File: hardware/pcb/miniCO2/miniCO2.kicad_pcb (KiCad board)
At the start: 4 copper layers, 13.7 x 28.2 mm, 12 parts, among them J1 USB_A, J2 Conn_01x04_Socket, SW1 SW_Push, U1 ATSAMD21E18A-M, U2 AP2112K-3.3, U3 SCD40-D-R2

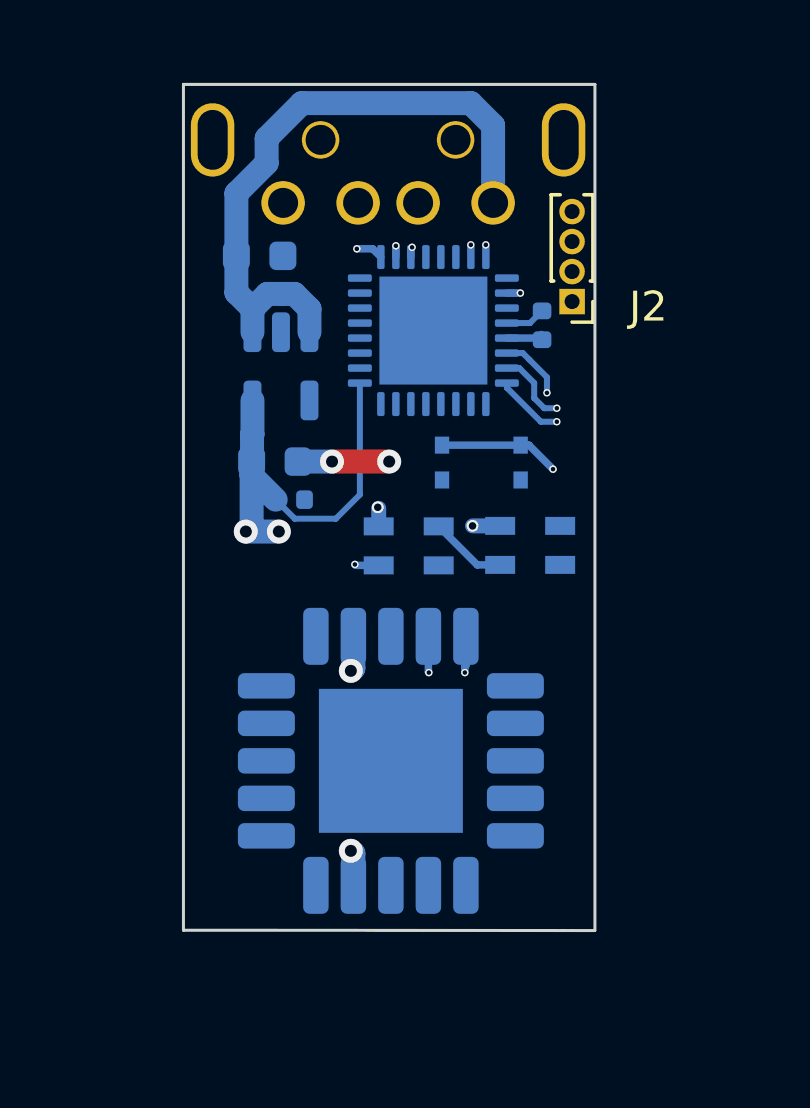
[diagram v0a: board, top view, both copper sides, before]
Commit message: Version 1 finished
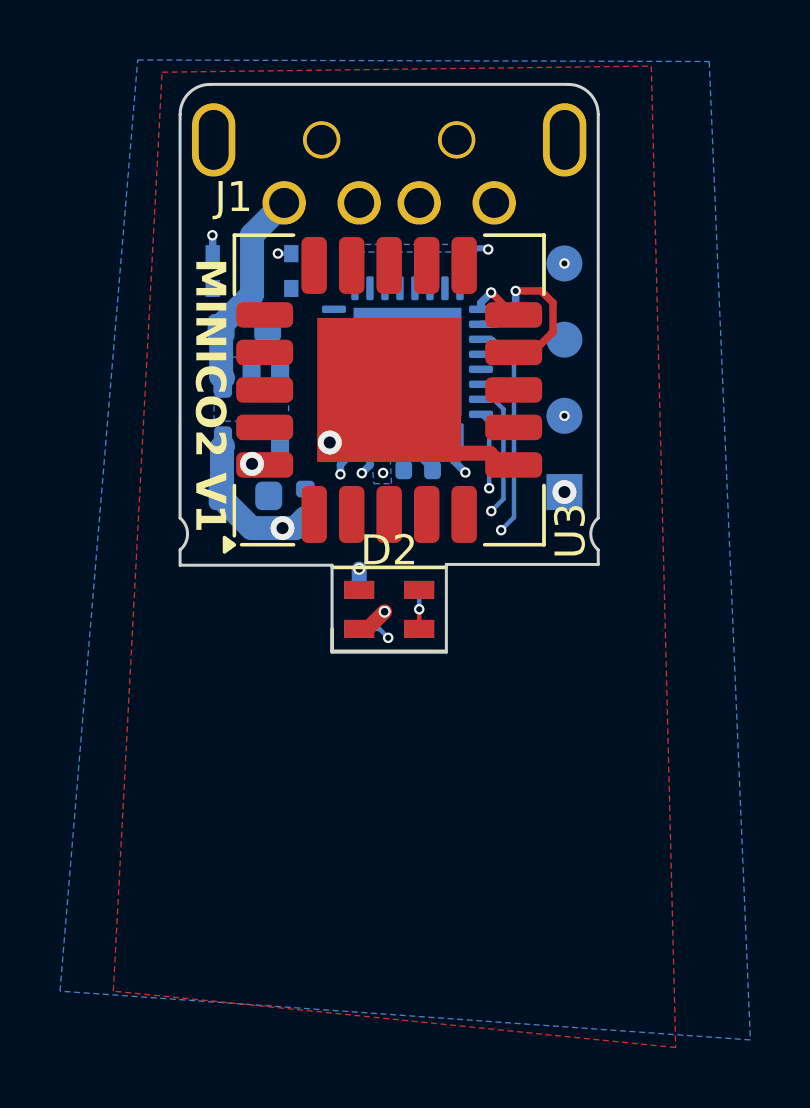
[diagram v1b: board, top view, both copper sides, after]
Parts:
- D1: footprint miniCO2:LED_SK6805_PLCC4_2.4x2.7mm_P1.3mm -> MiniCO2:LED_SK6805_PLCC4_2.4x2.7mm_P1.3mm
- D2: footprint miniCO2:LED_SK6805_PLCC4_2.4x2.7mm_P1.3mm -> MiniCO2:LED_SK6805_PLCC4_2.4x2.7mm_P1.3mm; moved to F.Cu
- J1: footprint miniCO2:917-P81A102ED60200 -> MiniCO2:917-P81A102ED60200; moved to F.Cu
- J2: footprint Connector_PinHeader_1.00mm:PinHeader_1x04_P1.00mm_Vertical -> MiniCO2:SWD_pogo_pads; moved to B.Cu
- SW1: footprint miniCO2:LS75C2D-T -> MiniCO2:LS75C2D-T
- U1: footprint miniCO2:QFN-32-1EP_5x5mm_P0.5mm_EP3.6x3.6mm -> MiniCO2:QFN-32-1EP_5x5mm_P0.5mm_EP3.6x3.6mm
- U3: footprint miniCO2:Sensirion_SCD4x-1EP_10.1x10.1mm_P1.25mm_EP4.8x4.8mm -> MiniCO2:Sensirion_SCD4x-1EP_10.1x10.1mm_P1.25mm_EP4.8x4.8mm; moved to F.Cu
- moved U3 12.4 mm to (141.5, 89.2), turned to 90 degrees
- moved SW1 9.96 mm to (136.9, 85.2)
- moved J2 6.36 mm to (147.3, 92.6), turned to 0 degrees
- moved C4 6.35 mm to (142.4, 91.8), turned to 180 degrees
- moved D2 5.16 mm to (141.5, 96.5), turned to 0 degrees
- moved C1 2.47 mm to (136.7, 87.1)
- moved D1 2.22 mm to (141.5, 96.5)
- moved U2 1.81 mm to (136.9, 89.9)
- moved C2 1.51 mm to (136.7, 92.7)
- moved U1 1.35 mm to (142.1, 88.2), turned to 0 degrees
- moved C3 0.52 mm to (138.7, 93.0), turned to -90 degrees
- turned J1 to 0 degrees
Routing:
- net SDA: track 17.8 -> 1.76 mm, vias 2 -> 1
- net D-: track 2.74 -> 17.7 mm
- net VBUS: track 21.1 -> 6.73 mm
- net SCL: track 19.1 -> 5.83 mm, vias 2 -> 1
- net Net-(U1-~{RESET}): track 10.8 -> 20.4 mm, vias 2 -> 3
- net +3.3V: track 20.4 -> 11.1 mm, vias 7 -> 5
- net D+: track 5.66 -> 14.8 mm
- net GND: track 4.38 -> 10.3 mm, vias 2 -> 3
- net DIN: track 12.5 -> 14.8 mm
- net SWDIO: track 8.59 -> 10.5 mm, vias 1 -> 2
- net SWCLK: track 10.3 -> 11.8 mm, vias 1 -> 2
- net Net-(D1-DOUT): track 2.58 -> 1.30 mm, vias 0 -> 1
- added copper zone on B.Cu, net +3.3V
- added copper zone on B.Cu, net VBUS
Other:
- board size 13.7 x 28.2 mm -> 13.9 x 18.9 mm
- board text added: "3.3"
- board text added: "CLK"
- board text added: "GND"
- board text added: "IO"
- board text added: "MINICO2 V1"
